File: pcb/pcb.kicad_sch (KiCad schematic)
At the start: 34 parts, among them J1 USB_C_Receptacle_USB2.0_16P, J2 TC2030_SWD, J3 Conn_01x02_MountingPin, J4 Conn_01x04_MountingPin, SW1 SW_SPDT, SW2 RST, SW3 Kailh_Choc, SW4 Kailh_Choc, SW5 Kailh_Choc, SW6 Kailh_Choc, SW7 Kailh_Choc, SW8 Kailh_Choc, U1 nRF52840_holyiot_18010, U2 SRV05-4, U3 TP4056, U4 XC6206PxxxMR

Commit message: finish footprint assignment
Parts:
- SW1: footprint (none) -> Button_Switch_SMD:SW_SPDT_PCM12
- SW2: footprint (none) -> Button_Switch_THT:SW_PUSH_6mm_H4.3mm
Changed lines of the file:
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@@
 			)
 		)
-		(property "Footprint" ""
+		(property "Footprint" "Button_Switch_SMD:SW_SPDT_PCM12"
 			(at 228.6 137.16 0)
 			(effects
@@
 			)
 		)
-		(property "Footprint" ""
+		(property "Footprint" "Button_Switch_THT:SW_PUSH_6mm_H4.3mm"
 			(at 27.94 77.47 0)
 			(effects

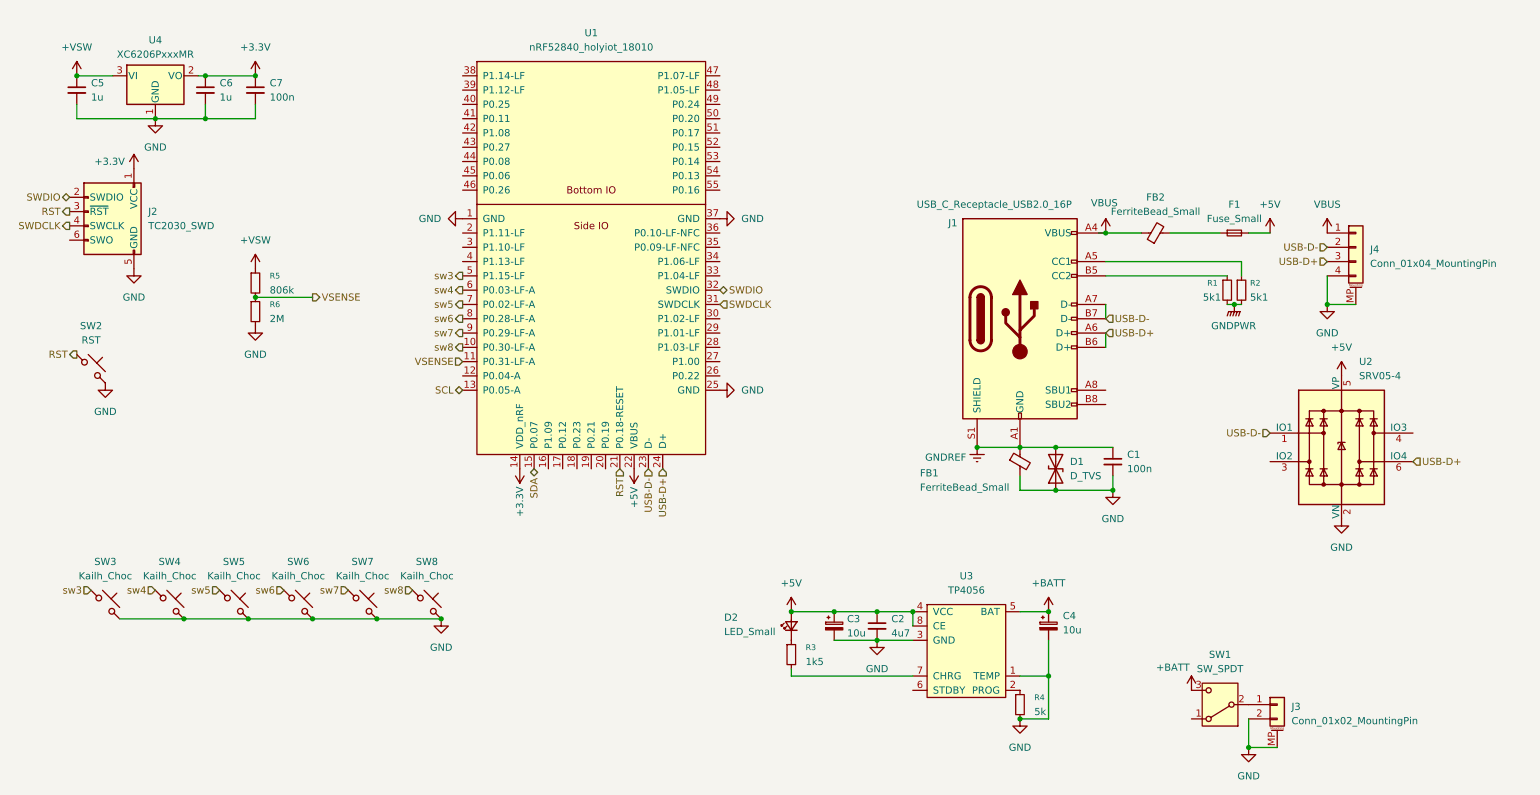
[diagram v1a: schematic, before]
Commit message: routing is hard
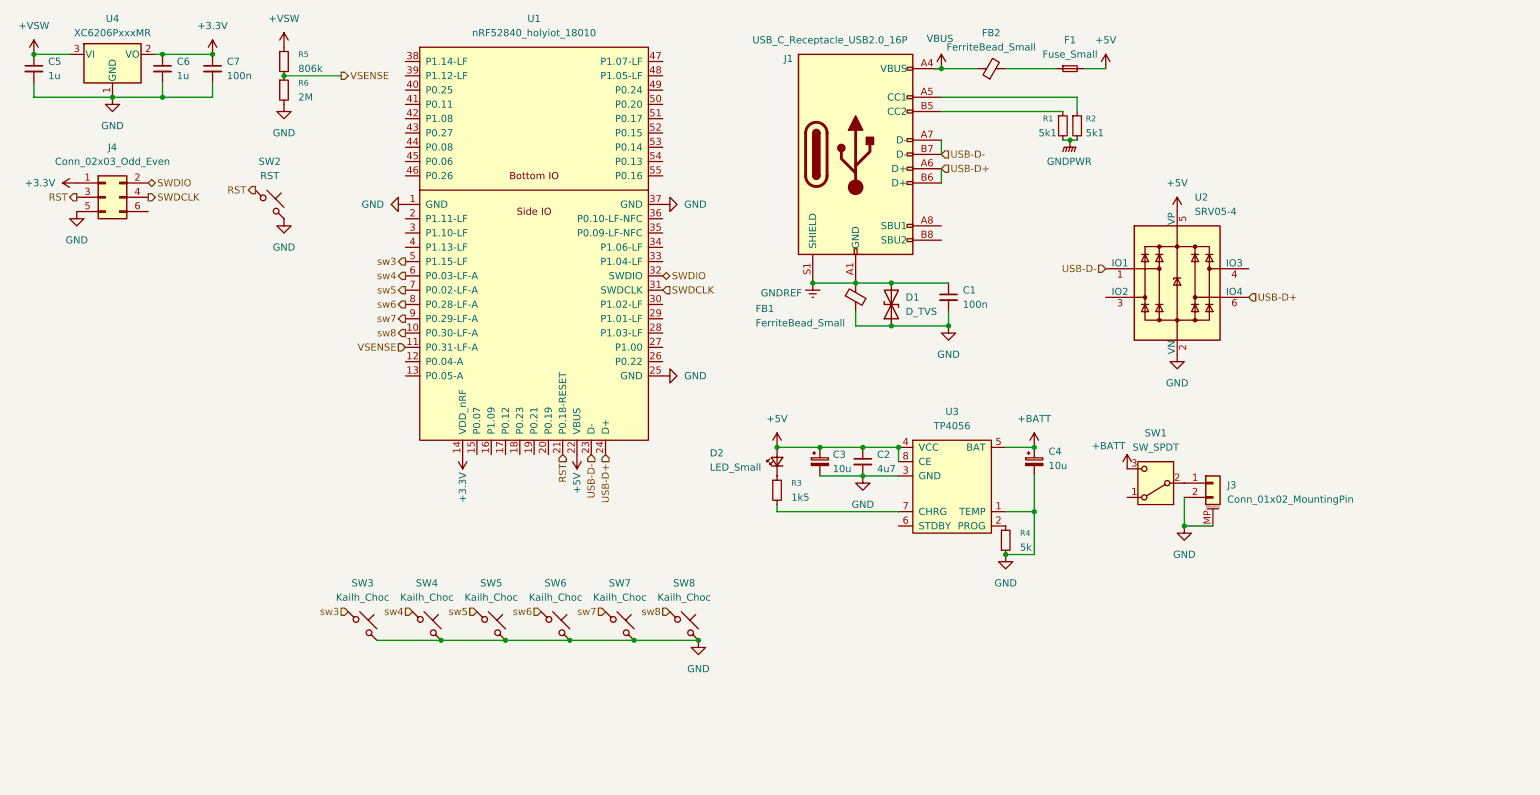
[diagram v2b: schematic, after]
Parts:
- removed J2: TC2030_SWD, PCM_marbastlib-various:CON_TC2030_outlined, symbol PCM_marbastlib-various:TC2030_SWD
- removed J4: Conn_01x04_MountingPin, Connector_JST:JST_SH_SM04B-SRSS-TB_1x04-1MP_P1.00mm_Horizontal, symbol Connector_Generic_MountingPin:Conn_01x04_MountingPin
- added J4: Conn_02x03_Odd_Even, Connector_PinHeader_2.54mm:PinHeader_2x03_P2.54mm_Vertical, symbol Connector_Generic:Conn_02x03_Odd_Even
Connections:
- net +3.3V: now also J4.1 (Pin_1)
- net GND: now also J4.5 (Pin_5)
- net RST: now also J4.3 (Pin_3)
- net SWDCLK: now also J4.4 (Pin_4)
- net SWDIO: now also J4.2 (Pin_2)
- net SCL: no longer names the net of U1.13 (P0.05-A)
- net SDA: no longer names the net of U1.15 (P0.07)
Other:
- moved on the sheet: C1, C2, C3, C4, C5, C6, C7, D1, D2, F1, FB1, FB2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
